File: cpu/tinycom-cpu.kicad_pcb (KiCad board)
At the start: 4 copper layers, 39.4 x 41.4 mm, 23 parts, among them P1 CONN_02X08, P2 CONN_02X08, U1 OLIMEX_IC_A13, U2 H5TQ2G83BFR/FBGA82, Y1 Crystal

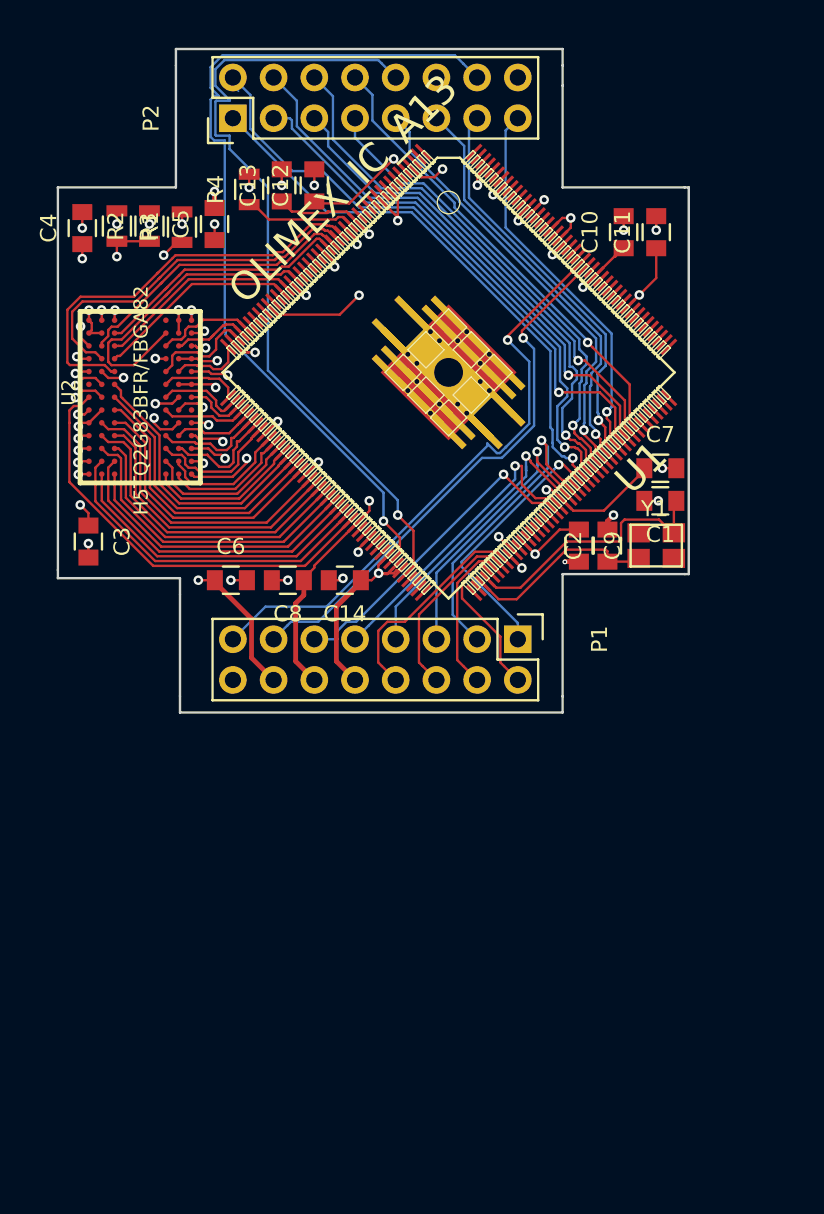
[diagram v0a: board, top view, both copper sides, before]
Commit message: adjust
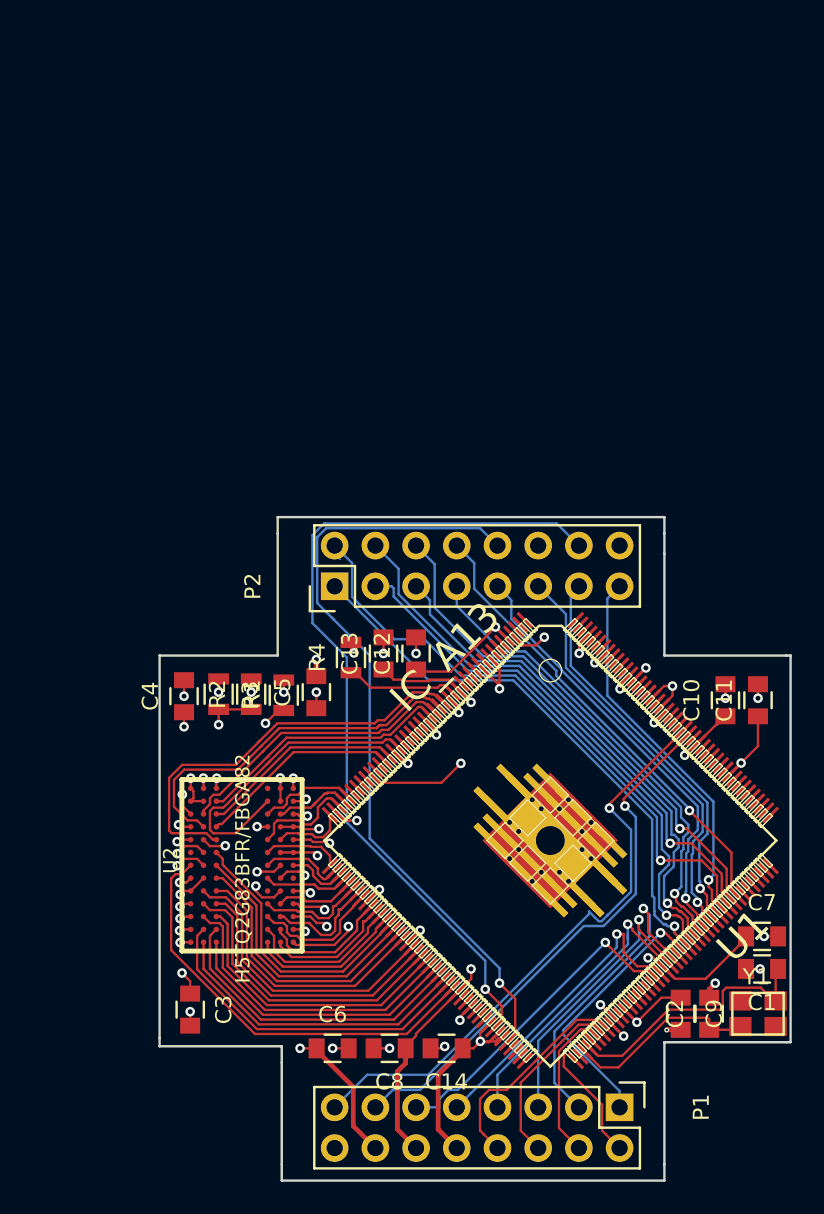
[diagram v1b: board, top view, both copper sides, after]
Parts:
- U1: value OLIMEX_IC_A13 -> IC_A13
- moved C1 29.9 mm to (122.9, 147.8)
- moved C14 29.9 mm to (103.3, 152.8)
- moved C2 29.9 mm to (119.6, 150.6)
- moved C4 29.9 mm to (86.9, 130.8)
- moved C5 29.9 mm to (95.1, 130.6)
- moved C6 29.9 mm to (96.1, 152.8)
- moved C8 29.9 mm to (99.7, 152.8)
- moved C9 29.9 mm to (117.9, 150.6)
- moved U1 29.9 mm to (109.7, 139.8)
- moved Y1 29.9 mm to (122.7, 150.6)
- moved C10 29.9 mm to (120.7, 131.1)
- moved C11 29.9 mm to (122.7, 131.1)
- moved C12 29.9 mm to (101.3, 128.1)
- moved C7 29.9 mm to (122.9, 145.8)
- moved P1 29.9 mm to (114.0, 156.5)
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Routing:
- net MICIN1: track 50.5 -> 49.0 mm
- net VCC_30: track 54.4 -> 53.4 mm
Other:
- net class Default: trace_width 0.3 -> 0.15
